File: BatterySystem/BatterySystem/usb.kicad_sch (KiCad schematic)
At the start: 1 part

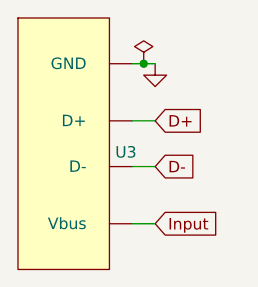
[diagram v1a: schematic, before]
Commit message: USB  connectie
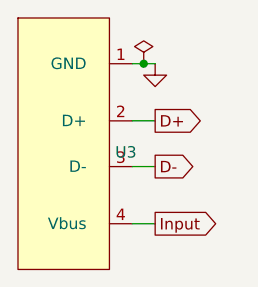
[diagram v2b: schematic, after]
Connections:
- net D+: now also U3.2 (D+); no longer U3. (Vbus)
- net D-: now also U3.3 (D-); no longer U3. (Vbus)
- net GND: now also U3.1 (GND); no longer U3. (Vbus)
- net Input: now also U3.4 (Vbus); no longer U3. (Vbus)
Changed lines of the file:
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@@
     (stroke (width 0) (type default))
   )
-  (global_label "Input" (shape input) (at 105.41 105.41 0) (fields_autoplaced)
+  (global_label "Input" (shape output) (at 105.41 105.41 0) (fields_autoplaced)
     (effects (font (size 1.27 1.27)) (justify left))
     (property "Intersheetrefs" "${INTERSHEET_REFS}" (at 113.0933 105.41 0)
@@
     )
   )
-  (global_label "D+" (shape input) (at 105.41 93.98 0) (fields_autoplaced)
+  (global_label "D+" (shape output) (at 105.41 93.98 0) (fields_autoplaced)
     (effects (font (size 1.27 1.27)) (justify left))
     (property "Intersheetrefs" "${INTERSHEET_REFS}" (at 111.1582 93.98 0)
@@
     )
   )
-  (global_label "D-" (shape input) (at 105.41 99.06 0) (fields_autoplaced)
+  (global_label "D-" (shape output) (at 105.41 99.06 0) (fields_autoplaced)
     (effects (font (size 1.27 1.27)) (justify left))
     (property "Intersheetrefs" "${INTERSHEET_REFS}" (at 111.1582 99.06 0)
@@
       (effects (font (size 1.27 1.27)) hide)
     )
-    (pin "")
-    (pin "")
-    (pin "")
-    (pin "")
+    (pin "2")
+    (pin "3")
+    (pin "1")
+    (pin "4")
     (instances
       (project "BatterySystem"
